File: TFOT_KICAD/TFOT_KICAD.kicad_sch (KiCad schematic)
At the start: 0 parts

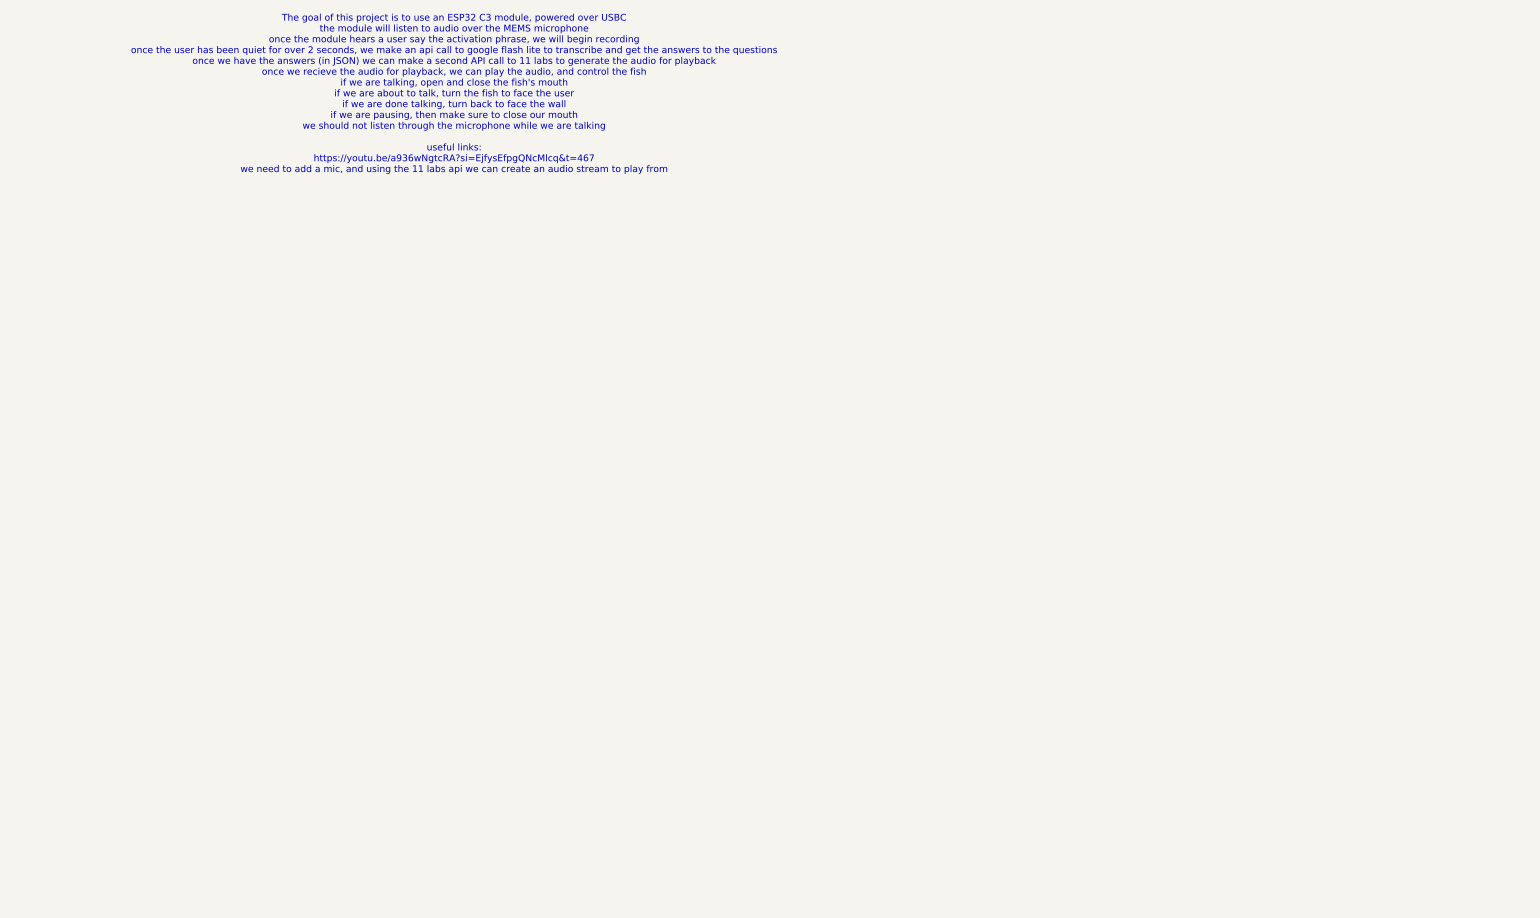
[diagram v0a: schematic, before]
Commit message: initial additions to board
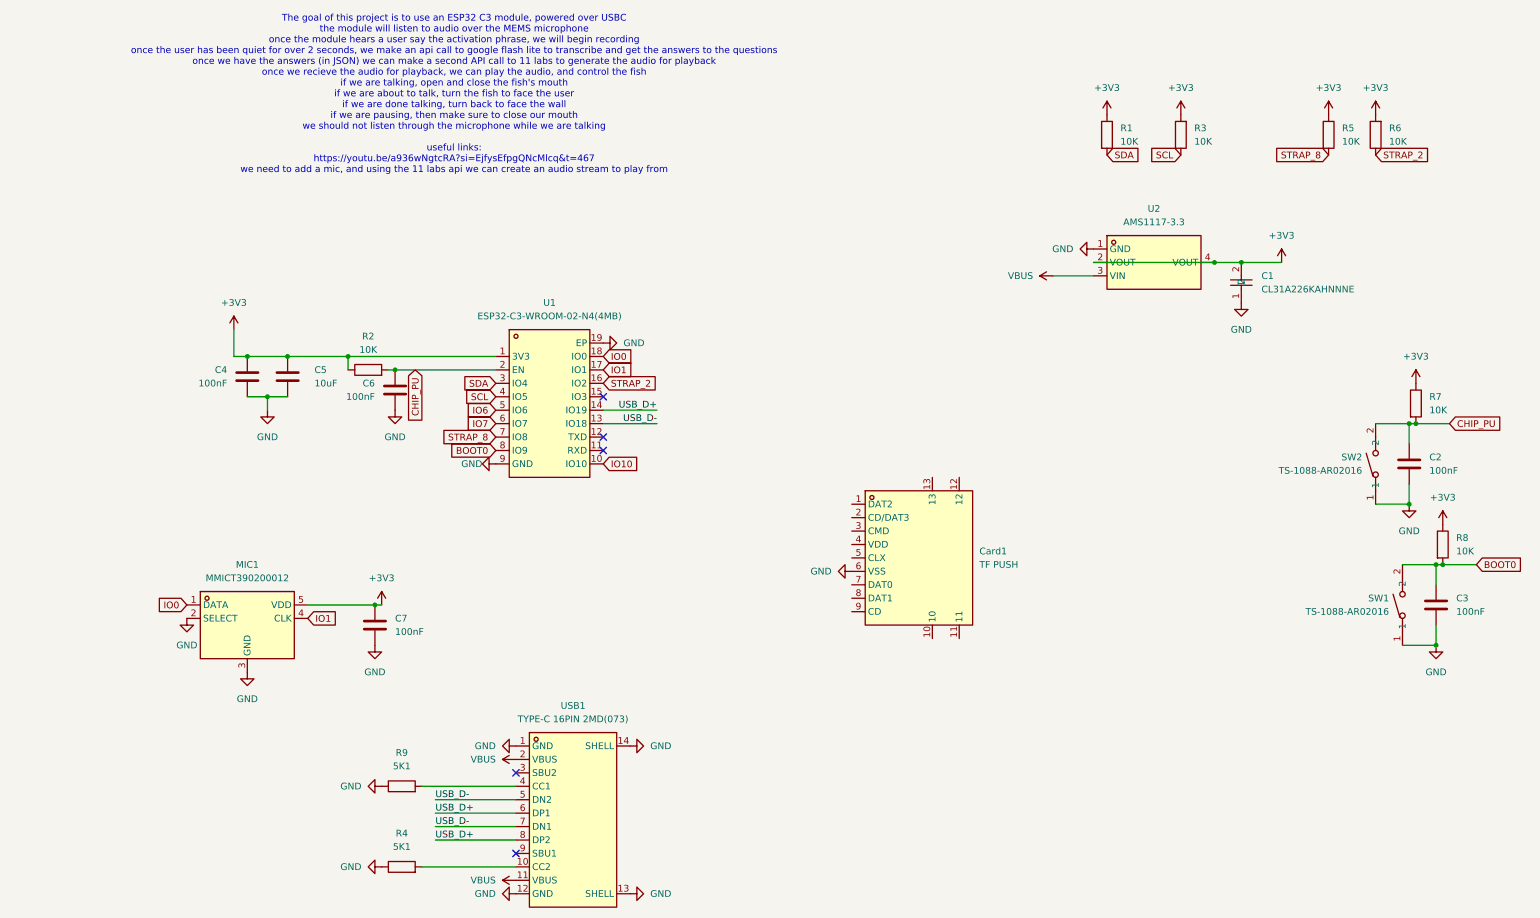
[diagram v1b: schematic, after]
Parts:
- added C1: CL31A226KAHNNNE, lib:C1206, symbol lib:CL31A226KAHNNNE
- added C2, C3, C4, C6: 100nF, Capacitor_SMD:C_0402_1005Metric, symbol Device:C
- added C5: 10uF, Capacitor_SMD:C_0603_1608Metric, symbol Device:C
- added C7: 100nF, symbol Device:C
- added Card1: TF PUSH, lib:TF-SMD_TF-PUSH, symbol lib:TFPUSH
- added MIC1: MMICT390200012, lib:MIC-SMD_5P-L3.5-W2.7-TL_MMICT390200012, symbol lib:MMICT390200012
- added R1, R2, R3, R5, R6, R7, R8: 10K, Resistor_SMD:R_0603_1608Metric, symbol Device:R
- added R4, R9: 5K1, symbol Device:R
- added SW1, SW2: TS-1088-AR02016, lib:SW-SMD_L3.9-W3.0-P4.45, symbol lib:TS-1088-AR02016
- added U1: ESP32-C3-WROOM-02-N4(4MB), lib:BULETM-SMD_ESPRESSIF_ESP32-C3-WROOM-02-N4-4MB, symbol lib:ESP32-C3-WROOM-02-N4(4MB)
- added U2: AMS1117-3.3, lib:SOT-223-3_L6.5-W3.4-P2.30-LS7.0-BR, symbol lib:AMS1117-3.3
- added USB1: TYPE-C 16PIN 2MD(073), lib:USB-C-SMD_TYPE-C-6PIN-2MD-073, symbol lib:TYPE-C16PIN2MD(073)
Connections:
- new net: R4.2, USB1.10 (CC2)
- new net: R9.2, USB1.4 (CC1)
- new net +3V3: C1.2, C4.1, C5.1, C7.1, MIC1.5 (VDD), R1.1, R2.1, R3.2, R5.1, R6.2, R7.1, R8.1, U1.1 (3V3), U2.2 (VOUT), U2.4 (VOUT)
- new net BOOT0: C3.1, R8.2, SW1.2, U1.8 (IO9)
- new net CHIP_PU: C2.1, C6.1, R2.2, R7.2, SW2.2, U1.2 (EN)
- new net GND: C1.1, C2.2, C3.2, C4.2, C5.2, C6.2, C7.2, Card1.6 (VSS), MIC1.2 (SELECT), MIC1.3 (GND), R4.1, R9.1, SW1.1, SW2.1, U1.19 (EP), U1.9 (GND), U2.1 (GND), USB1.1 (GND), USB1.12 (GND), USB1.13 (SHELL), USB1.14 (SHELL)
- new net IO0: MIC1.1 (DATA), U1.18 (IO0)
- new net IO1: MIC1.4 (CLK), U1.17 (IO1)
- new net IO10: U1.10 (IO10)
- new net IO6: U1.5 (IO6)
- new net IO7: U1.6 (IO7)
- new net SCL: R3.1, U1.4 (IO5)
- new net SDA: R1.2, U1.3 (IO4)
- new net STRAP_2: R6.1, U1.16 (IO2)
- new net STRAP_8: R5.2, U1.7 (IO8)
- new net USB_D+: U1.14 (IO19), USB1.6 (DP1), USB1.8 (DP2)
- new net USB_D-: U1.13 (IO18), USB1.5 (DN2), USB1.7 (DN1)
- new net VBUS: U2.3 (VIN), USB1.11 (VBUS), USB1.2 (VBUS)
- no-connect marks 0 -> 5
